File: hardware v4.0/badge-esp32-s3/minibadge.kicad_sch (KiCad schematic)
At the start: 15 parts, among them J12 Conn_01x02_Socket, J13 Conn_01x04_Socket, J5 Conn_01x02_Socket, J6 Conn_01x04_Socket, J7 Conn_01x08_Socket, J8 Conn_01x08_Socket, J9 Conn_02x06_Odd_Even

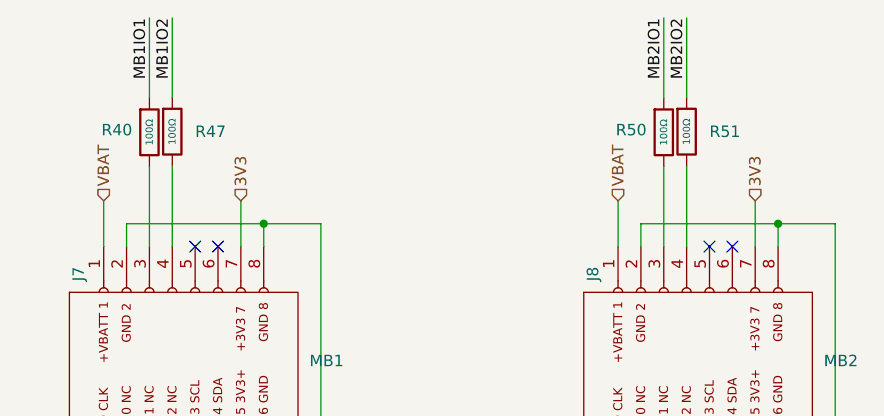
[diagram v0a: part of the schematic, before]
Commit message: finished schematics and layout
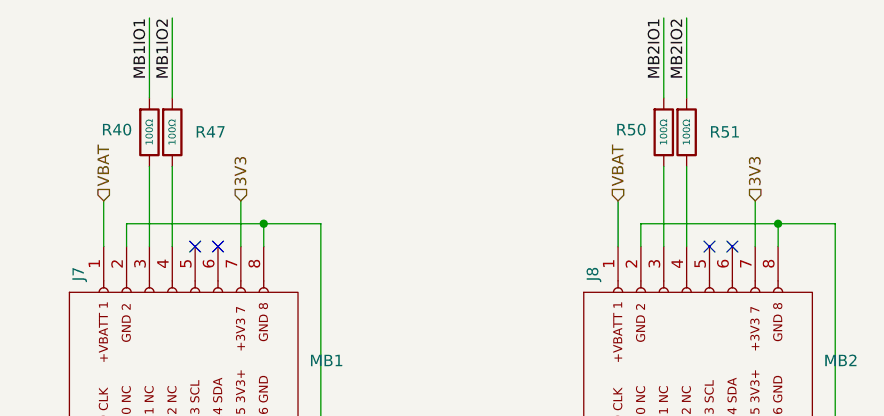
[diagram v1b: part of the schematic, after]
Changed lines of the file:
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@@
 	(wire
 		(pts
-			(xy 160.02 53.2702) (xy 160.02 62.23)
+			(xy 160.02 53.34) (xy 160.02 62.23)
 		)
 		(stroke
@@
 	(wire
 		(pts
-			(xy 102.87 36.83) (xy 102.87 45.6502)
+			(xy 102.87 36.83) (xy 102.87 45.72)
 		)
 		(stroke
@@
 	(wire
 		(pts
-			(xy 102.87 53.2702) (xy 102.87 62.23)
+			(xy 102.87 53.34) (xy 102.87 62.23)
 		)
 		(stroke
@@
 	(wire
 		(pts
-			(xy 160.02 36.83) (xy 160.02 45.6502)
+			(xy 160.02 36.83) (xy 160.02 45.72)
 		)
 		(stroke
@@
 	(symbol
 		(lib_id "PCM_JLCPCB-Resistors:0402,100Ω")
-		(at 160.02 49.4602 0)
+		(at 160.02 49.53 0)
 		(unit 1)
 		(exclude_from_sim no)
@@
 		(fields_autoplaced yes)
 		(property "Reference" "R51"
-			(at 162.56 49.4601 0)
+			(at 162.56 49.5299 0)
 			(effects
 				(font
@@
 		)
 		(property "Value" "100Ω"
-			(at 160.02 49.4602 90)
+			(at 160.02 49.53 90)
 			(do_not_autoplace yes)
 			(effects
@@
 		)
 		(property "Footprint" "PCM_JLCPCB:R_0402"
-			(at 158.242 49.4602 90)
+			(at 158.242 49.53 90)
 			(effects
 				(font
@@
 		)
 		(property "Datasheet" "https://www.lcsc.com/datasheet/lcsc_datasheet_2205311900_UNI-ROYAL-Uniroyal-Elec-0402WGF1000TCE_C25076.pdf"
-			(at 160.02 49.4602 0)
+			(at 160.02 49.53 0)
 			(effects
 				(font
@@
 		)
 		(property "Description" "62.5mW Thick Film Resistors 50V ±1% ±200ppm/°C 100Ω 0402 Chip Resistor - Surface Mount ROHS"
-			(at 160.02 49.4602 0)
+			(at 160.02 49.53 0)
 			(effects
 				(font
@@
 		)
 		(property "LCSC" "C25076"
-			(at 160.02 49.4602 0)
+			(at 160.02 49.53 0)
 			(effects
 				(font
@@
 		)
 		(property "Stock" "5907585"
-			(at 160.02 49.4602 0)
+			(at 160.02 49.53 0)
 			(effects
 				(font
@@
 		)
 		(property "Price" "0.004USD"
-			(at 160.02 49.4602 0)
+			(at 160.02 49.53 0)
 			(effects
 				(font
@@
 		)
 		(property "Process" "SMT"
-			(at 160.02 49.4602 0)
+			(at 160.02 49.53 0)
 			(effects
 				(font
@@
 		)
 		(property "Minimum Qty" "20"
-			(at 160.02 49.4602 0)
+			(at 160.02 49.53 0)
 			(effects
 				(font
@@
 		)
 		(property "Attrition Qty" "10"
-			(at 160.02 49.4602 0)
+			(at 160.02 49.53 0)
 			(effects
 				(font
@@
 		)
 		(property "Class" "Basic Component"
-			(at 160.02 49.4602 0)
+			(at 160.02 49.53 0)
 			(effects
 				(font
@@
 		)
 		(property "Category" "Resistors,Chip Resistor - Surface Mount"
-			(at 160.02 49.4602 0)
+			(at 160.02 49.53 0)
 			(effects
 				(font
@@
 		)
 		(property "Manufacturer" "UNI-ROYAL(Uniroyal Elec)"
-			(at 160.02 49.4602 0)
+			(at 160.02 49.53 0)
 			(effects
 				(font
@@
 		)
 		(property "Part" "0402WGF1000TCE"
-			(at 160.02 49.4602 0)
+			(at 160.02 49.53 0)
 			(effects
 				(font
@@
 		)
 		(property "Resistance" "100Ω"
-			(at 160.02 49.4602 0)
+			(at 160.02 49.53 0)
 			(effects
 				(font
@@
 		)
 		(property "Power(Watts)" "62.5mW"
-			(at 160.02 49.4602 0)
+			(at 160.02 49.53 0)
 			(effects
 				(font
@@
 		)
 		(property "Type" "Thick Film Resistors"
-			(at 160.02 49.4602 0)
+			(at 160.02 49.53 0)
 			(effects
 				(font
@@
 		)
 		(property "Overload Voltage (Max)" "50V"
-			(at 160.02 49.4602 0)
+			(at 160.02 49.53 0)
 			(effects
 				(font
@@
 		)
 		(property "Operating Temperature Range" "-55°C~+155°C"
-			(at 160.02 49.4602 0)
+			(at 160.02 49.53 0)
 			(effects
 				(font
@@
 		)
 		(property "Tolerance" "±1%"
-			(at 160.02 49.4602 0)
+			(at 160.02 49.53 0)
 			(effects
 				(font
@@
 		)
 		(property "Temperature Coefficient" "±200ppm/°C"
-			(at 160.02 49.4602 0)
+			(at 160.02 49.53 0)
 			(effects
 				(font
@@
 	(symbol
 		(lib_id "PCM_JLCPCB-Resistors:0402,100Ω")
-		(at 102.87 49.4602 0)
+		(at 102.87 49.53 0)
 		(unit 1)
 		(exclude_from_sim no)
@@
 		(fields_autoplaced yes)
 		(property "Reference" "R47"
-			(at 105.41 49.4601 0)
+			(at 105.41 49.5299 0)
 			(effects
 				(font
@@
 		)
 		(property "Value" "100Ω"
-			(at 102.87 49.4602 90)
+			(at 102.87 49.53 90)
 			(do_not_autoplace yes)
 			(effects
@@
 		)
 		(property "Footprint" "PCM_JLCPCB:R_0402"
-			(at 101.092 49.4602 90)
+			(at 101.092 49.53 90)
 			(effects
 				(font
@@
 		)
 		(property "Datasheet" "https://www.lcsc.com/datasheet/lcsc_datasheet_2205311900_UNI-ROYAL-Uniroyal-Elec-0402WGF1000TCE_C25076.pdf"
-			(at 102.87 49.4602 0)
+			(at 102.87 49.53 0)
 			(effects
 				(font
@@
 		)
 		(property "Description" "62.5mW Thick Film Resistors 50V ±1% ±200ppm/°C 100Ω 0402 Chip Resistor - Surface Mount ROHS"
-			(at 102.87 49.4602 0)
+			(at 102.87 49.53 0)
 			(effects
 				(font
@@
 		)
 		(property "LCSC" "C25076"
-			(at 102.87 49.4602 0)
+			(at 102.87 49.53 0)
 			(effects
 				(font
@@
 		)
 		(property "Stock" "5907585"
-			(at 102.87 49.4602 0)
+			(at 102.87 49.53 0)
 			(effects
 				(font
@@
 		)
 		(property "Price" "0.004USD"
-			(at 102.87 49.4602 0)
+			(at 102.87 49.53 0)
 			(effects
 				(font
@@
 		)
 		(property "Process" "SMT"
-			(at 102.87 49.4602 0)
+			(at 102.87 49.53 0)
 			(effects
 				(font
@@
 		)
 		(property "Minimum Qty" "20"
-			(at 102.87 49.4602 0)
+			(at 102.87 49.53 0)
 			(effects
 				(font
@@
 		)
 		(property "Attrition Qty" "10"
-			(at 102.87 49.4602 0)
+			(at 102.87 49.53 0)
 			(effects
 				(font
@@
 		)
 		(property "Class" "Basic Component"
-			(at 102.87 49.4602 0)
+			(at 102.87 49.53 0)
 			(effects
 				(font
@@
 		)
 		(property "Category" "Resistors,Chip Resistor - Surface Mount"
-			(at 102.87 49.4602 0)
+			(at 102.87 49.53 0)
 			(effects
 				(font
@@
 		)
 		(property "Manufacturer" "UNI-ROYAL(Uniroyal Elec)"
-			(at 102.87 49.4602 0)
+			(at 102.87 49.53 0)
 			(effects
 				(font
@@
 		)
 		(property "Part" "0402WGF1000TCE"
-			(at 102.87 49.4602 0)
+			(at 102.87 49.53 0)
 			(effects
 				(font
@@
 		)
 		(property "Resistance" "100Ω"
-			(at 102.87 49.4602 0)
+			(at 102.87 49.53 0)
 			(effects
 				(font
@@
 		)
 		(property "Power(Watts)" "62.5mW"
-			(at 102.87 49.4602 0)
+			(at 102.87 49.53 0)
 			(effects
 				(font
@@
 		)
 		(property "Type" "Thick Film Resistors"
-			(at 102.87 49.4602 0)
+			(at 102.87 49.53 0)
 			(effects
 				(font
@@
 		)
 		(property "Overload Voltage (Max)" "50V"
-			(at 102.87 49.4602 0)
+			(at 102.87 49.53 0)
 			(effects
 				(font
@@
 		)
 		(property "Operating Temperature Range" "-55°C~+155°C"
-			(at 102.87 49.4602 0)
+			(at 102.87 49.53 0)
 			(effects
 				(font
@@
 		)
 		(property "Tolerance" "±1%"
-			(at 102.87 49.4602 0)
+			(at 102.87 49.53 0)
 			(effects
 				(font
@@
 		)
 		(property "Temperature Coefficient" "±200ppm/°C"
-			(at 102.87 49.4602 0)
-			(effects
-				(font
+			(at 102.87 49.53 0)
+			(effects
+				(font
